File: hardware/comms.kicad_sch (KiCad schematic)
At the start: 1 part

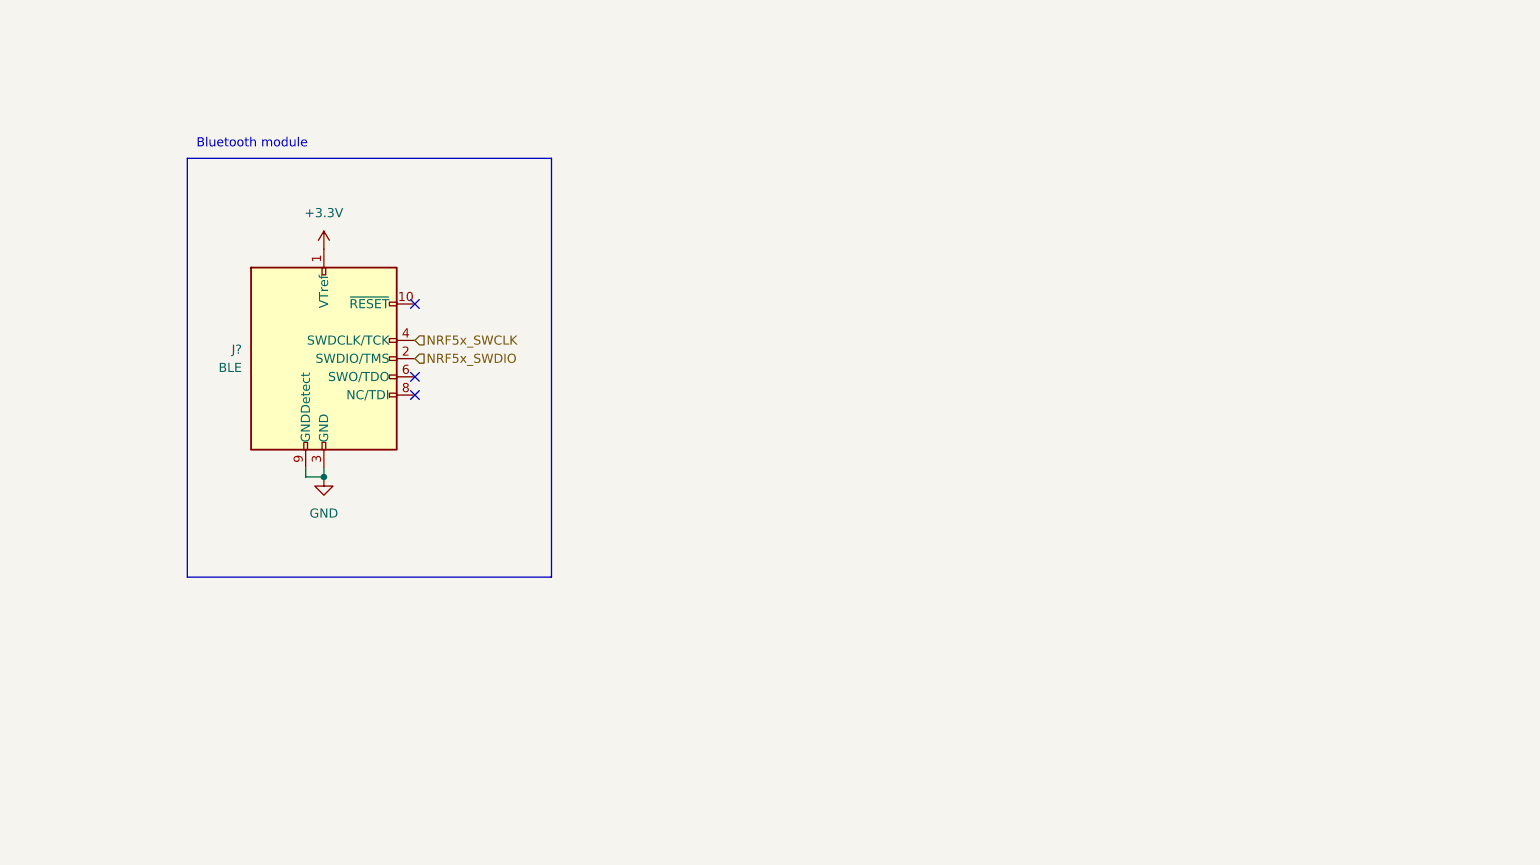
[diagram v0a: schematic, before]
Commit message: Communication interfaces
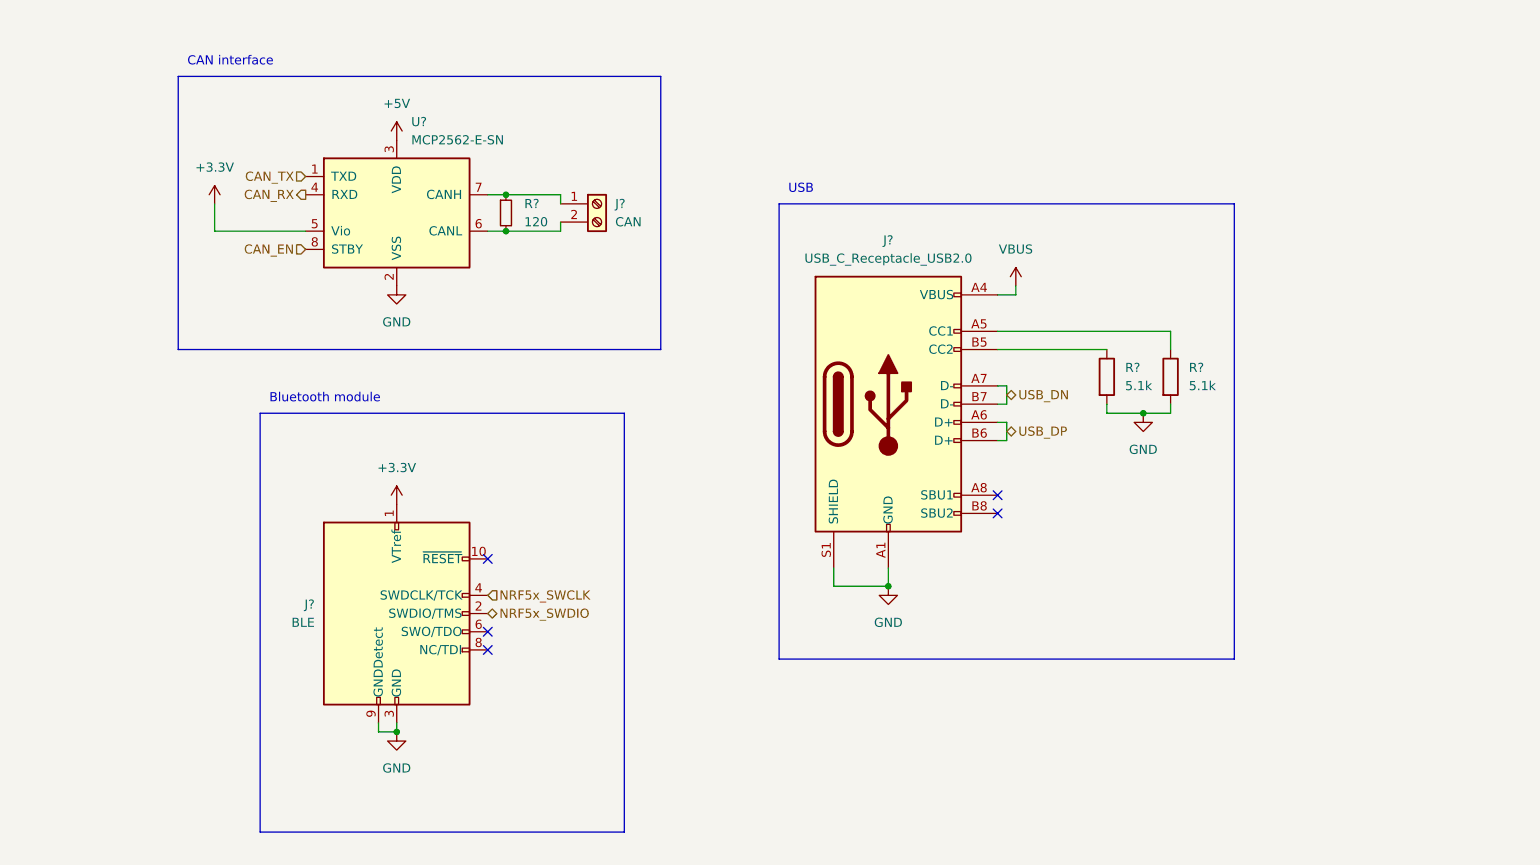
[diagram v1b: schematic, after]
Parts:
- added J?: USB_C_Receptacle_USB2.0, symbol Connector:USB_C_Receptacle_USB2.0
- added J?: CAN, symbol Connector:Screw_Terminal_01x02
- added R?: 120, symbol Device:R_Small
- added R? (x2): 5.1k, symbol Device:R
- added U?: MCP2562-E-SN, Package_SO:SOIC-8_3.9x4.9mm_P1.27mm, symbol Interface_CAN_LIN:MCP2562-E-SN
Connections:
- net +3.3V: now also U?.5 (Vio)
- net GND: now also J?.A1 (GND), J?.A12 (GND), J?.B1 (GND), J?.B12 (GND), J?.S1 (SHIELD), R?.2, R?.2, U?.2 (VSS)
- new net: J?.A5 (CC1), R?.1
- new net: J?.B5 (CC2), R?.1
- new net: J?.1 (Pin_1), R?.1, U?.7 (CANH)
- new net: J?.2 (Pin_2), R?.2, U?.6 (CANL)
- new net +5V: U?.3 (VDD)
- new net CAN_EN: U?.8 (STBY)
- new net CAN_RX: U?.4 (RXD)
- new net CAN_TX: U?.1 (TXD)
- new net USB_DN: J?.A7 (D-), J?.B7 (D-)
- new net USB_DP: J?.A6 (D+), J?.B6 (D+)
- new net VBUS: J?.A4 (VBUS), J?.A9 (VBUS), J?.B4 (VBUS), J?.B9 (VBUS)
- no-connect marks 3 -> 5
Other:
- note added: "CAN interface"
- note added: "USB"
- moved on the sheet: J?

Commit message: BLE module
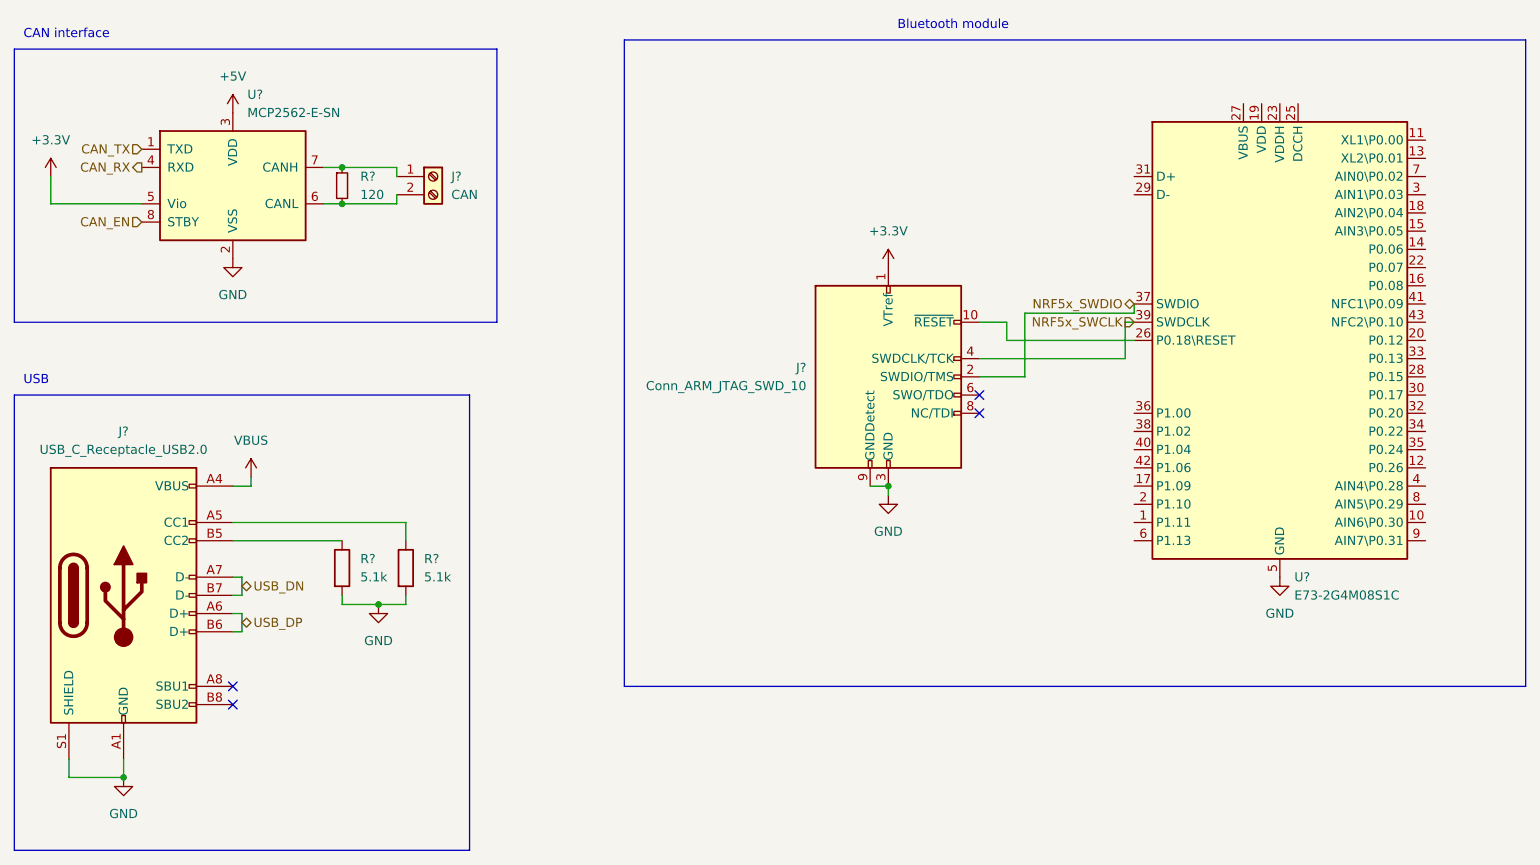
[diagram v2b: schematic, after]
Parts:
- removed J?: BLE, symbol Connector:Conn_ARM_JTAG_SWD_10
- added J?: Conn_ARM_JTAG_SWD_10, symbol Connector:Conn_ARM_JTAG_SWD_10
- added U?: E73-2G4M08S1C, vesc-bms:E73-2G4M08S1C, symbol vesc-bms:E73-2G4M08S1C
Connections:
- net +3.3V: now also J?.1 (VTref)
- net GND: now also J?.3 (GND), J?.5 (GND), J?.9 (GNDDetect), U?.21 (GND), U?.24 (GND), U?.5 (GND)
- net NRF5x_SWCLK: now also J?.4 (SWDCLK/TCK), U?.39 (SWDCLK)
- net NRF5x_SWDIO: now also J?.2 (SWDIO/TMS), U?.37 (SWDIO)
- new net: J?.10 (~{RESET}), U?.26 (P0.18\RESET)
- no-connect marks 5 -> 4
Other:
- moved on the sheet: J?, R?, U?
